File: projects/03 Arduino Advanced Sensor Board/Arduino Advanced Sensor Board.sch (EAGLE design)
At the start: 40 parts

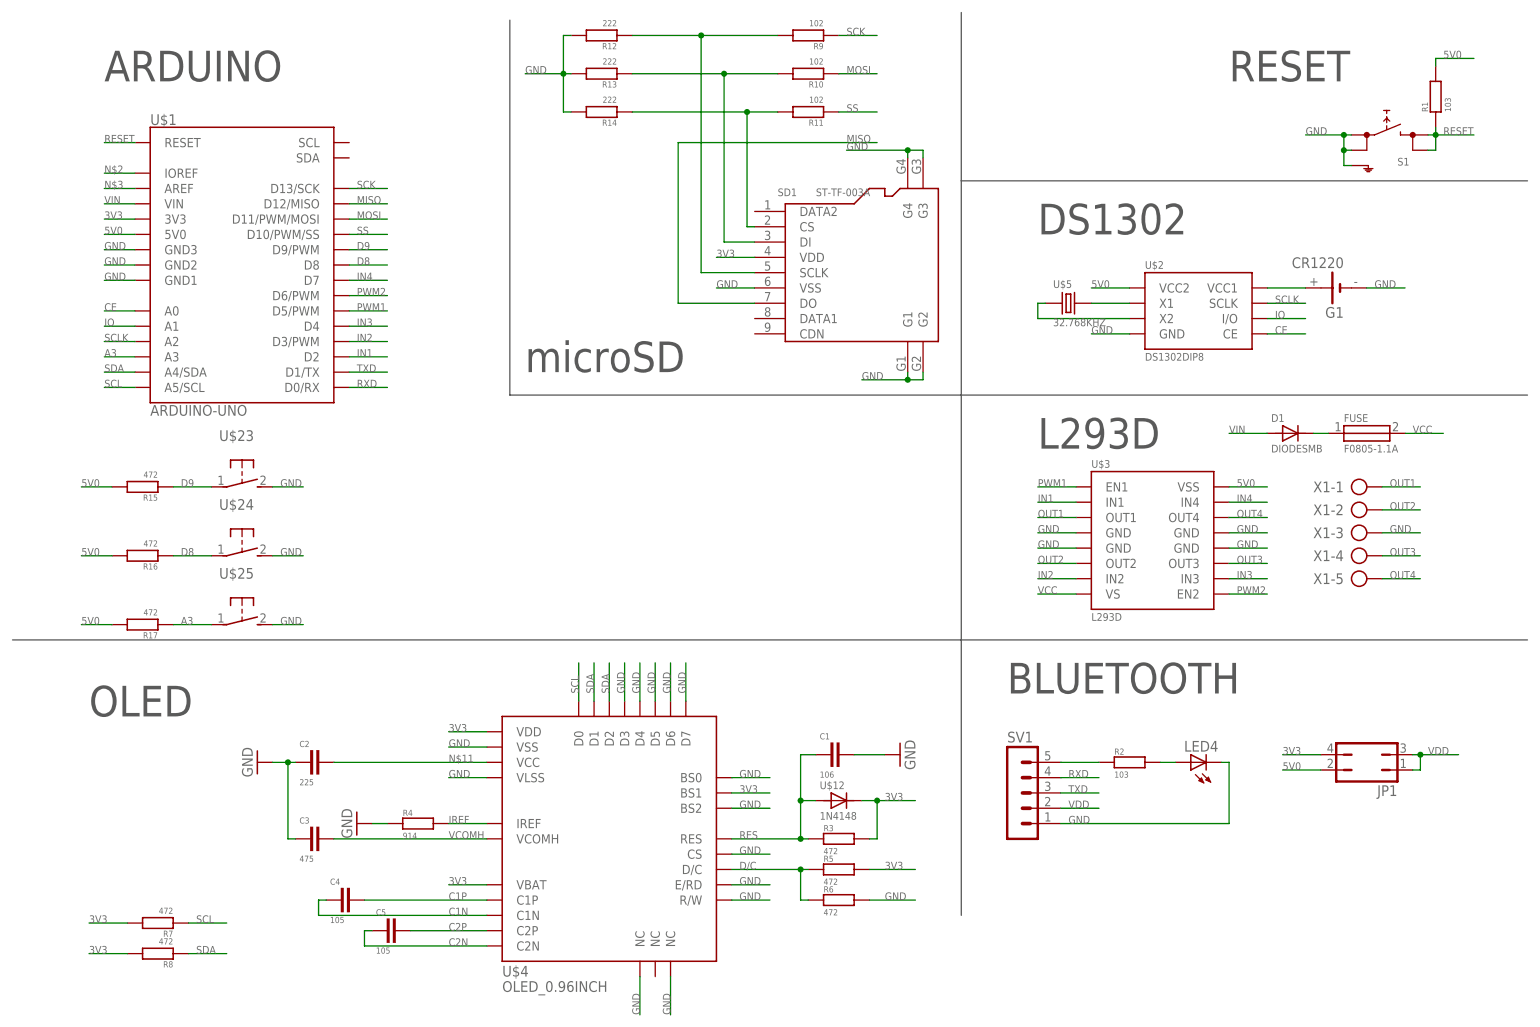
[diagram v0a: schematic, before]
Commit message: 2020.07.02.01
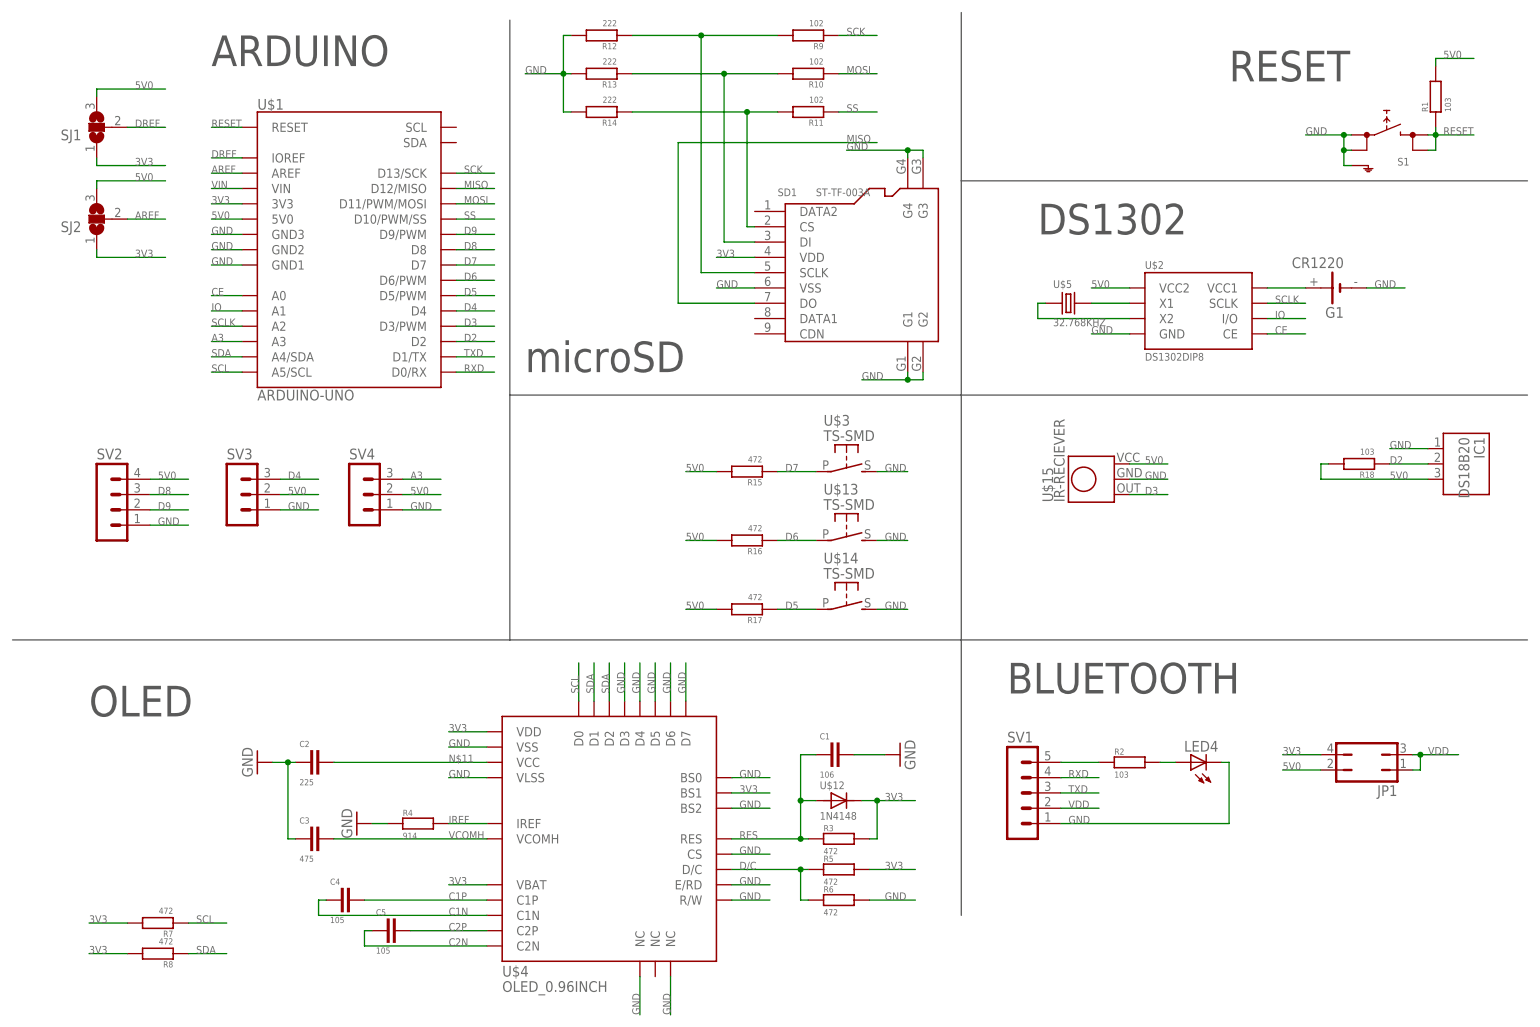
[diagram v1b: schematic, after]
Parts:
- removed D1: DIODESMB, RCLDA:DIODESMB
- removed FUSE: F0805-1.1A, RCLDA:FUSE0805
- removed U$23, U$24, U$25: TS-SMD_36TS-SMD-3*6, Button:TS-SMD_36TS-SMD-3*6
- removed X1: (no value), Connector:AK500/5
- added IC1: DS18B20, Senser:DS18B20
- added R18: 103, RCLDA:R0805
- added SJ1, SJ2: (no value), Jumper:SJ2W
- added SV2: (no value), Pin-Header:MA04-1
- added SV3, SV4: (no value), Pin-Header:MA03-1
- added U$13, U$14: TS-SMD, Button:TS-SMD
- added U$15: IR-RECIEVER, Senser:IR-RECIEVER
- U$3: value L293D -> TS-SMD; device Chip:L293D -> Button:TS-SMD
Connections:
- removed net IN1: U$1.D2, U$3.IN1
- removed net IN2: U$1.D3/PWM, U$3.IN2
- removed net IN3: U$1.D4, U$3.IN3
- removed net IN4: U$1.D7, U$3.IN4
- removed net N$1: D1.1, FUSE.P$1
- removed net N$2: U$1.IOREF
- removed net N$3: U$1.AREF
- removed net OUT1: U$3.OUT1, X1-1.KL
- removed net OUT2: U$3.OUT2, X1-2.KL
- removed net OUT3: U$3.OUT3, X1-4.KL
- removed net OUT4: U$3.OUT4, X1-5.KL
- removed net PWM1: U$1.D5/PWM, U$3.EN1
- removed net PWM2: U$1.D6/PWM, U$3.EN2
- removed net VCC: FUSE.P$2, U$3.VS
- new net AREF: SJ2.2, U$1.AREF
- new net D2: IC1.DQ, R18.1, U$1.D2
- new net D3: U$1.D3/PWM, U$15.OUT
- new net D4: SV3.3, U$1.D4
- new net D5: R17.1, U$1.D5/PWM, U$14.P
- new net D6: R16.1, U$1.D6/PWM, U$13.P
- new net D7: R15.1, U$1.D7, U$3.P
- new net DREF: SJ1.2, U$1.IOREF
- net 3V3: now also SJ1.1, SJ2.1
- net 5V0: now also IC1.VCC, R18.2, SJ1.3, SJ2.3, SV2.4, SV3.2, SV4.2, U$15.VCC; no longer U$3.VSS
- net A3: now also SV4.3; no longer R17.1, U$25.P
- net D8: now also SV2.3; no longer R16.1, U$24.P
- net D9: now also SV2.2; no longer R15.1, U$23.P
- net GND: now also IC1.GND, SV2.1, SV3.1, SV4.1, U$13.S, U$14.S, U$15.GND, U$3.S; no longer U$23.S, U$24.S, U$25.S, U$3.GND@1, U$3.GND@2, U$3.GND@3, U$3.GND@4, X1-3.KL
- net VIN: no longer D1.2
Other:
- note removed: "L293D"
- moved on the sheet: R15, R16, R17, U$1
